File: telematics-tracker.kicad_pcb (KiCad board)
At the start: 4 copper layers, 82 x 62 mm, 216 parts, among them J1 WAFER-MX3.0-12PZZ, J2 B3B-XH-A, Q1 AM2390N-TP, Q10 MMBT3904, Q11 MMBT3904, Q12 MMBT3904, Q13 MMBT3906, Q14 MMBT3904, Q2 AM2390N-TP, Q3 AO3401A, Q4 MMBT3904, Q5 MMBT3904, Q6 MMBT3904, Q7 MMBT3904, Q8 MMBT3904, Q9 MMBT3904, U1 EC200UCNAA-N05-SGNSA, U2 AT32F403ACGT7, U3 QMI8658B, U4 SIT1051AT/3, U5 EG11752, U6 BQ25606RGER, U7 GD25Q64ESIGR, U8 TXB0104PWR, U9 ME6211C33M5G, X1 NANO-SIM, X2 MFF2-eSIM-pads, Y1 8MHz, Y2 32.768kHz

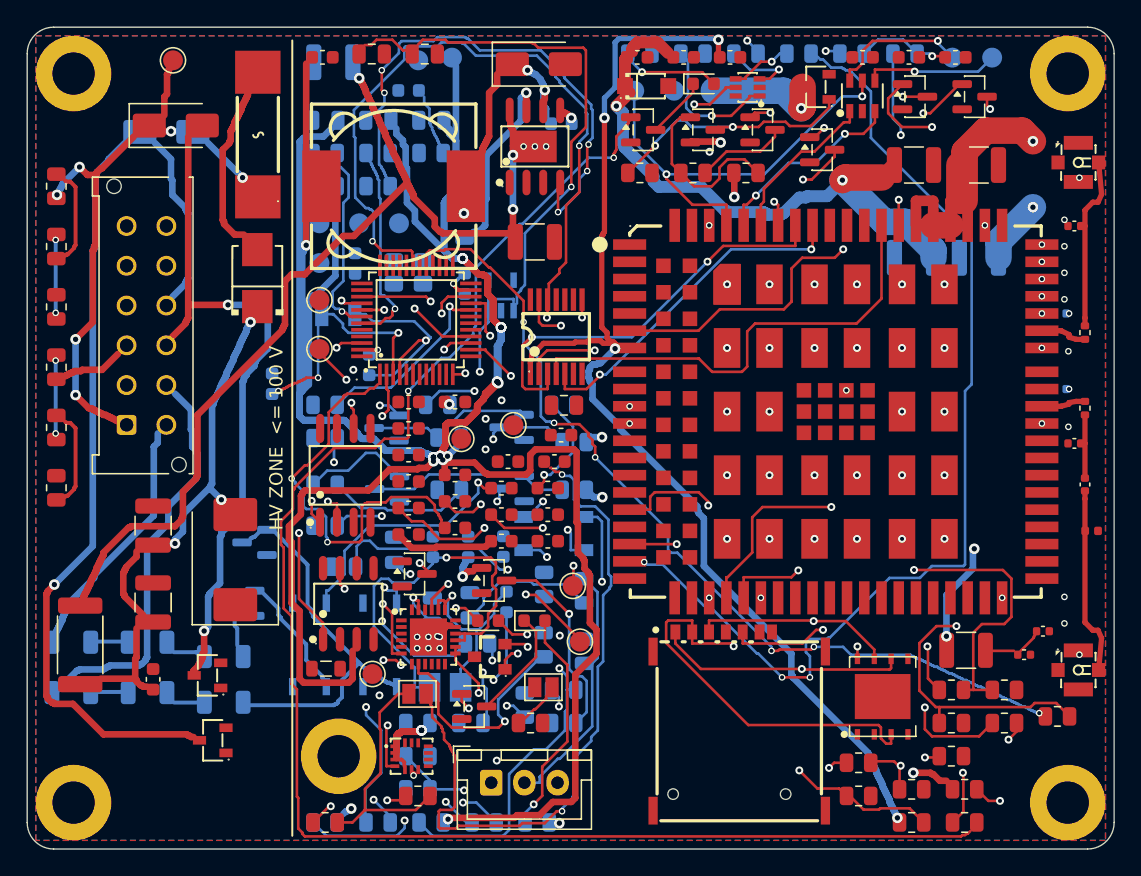
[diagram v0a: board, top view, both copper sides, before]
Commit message: hybrid v11 cycle 1: unconnected=150 errors=0
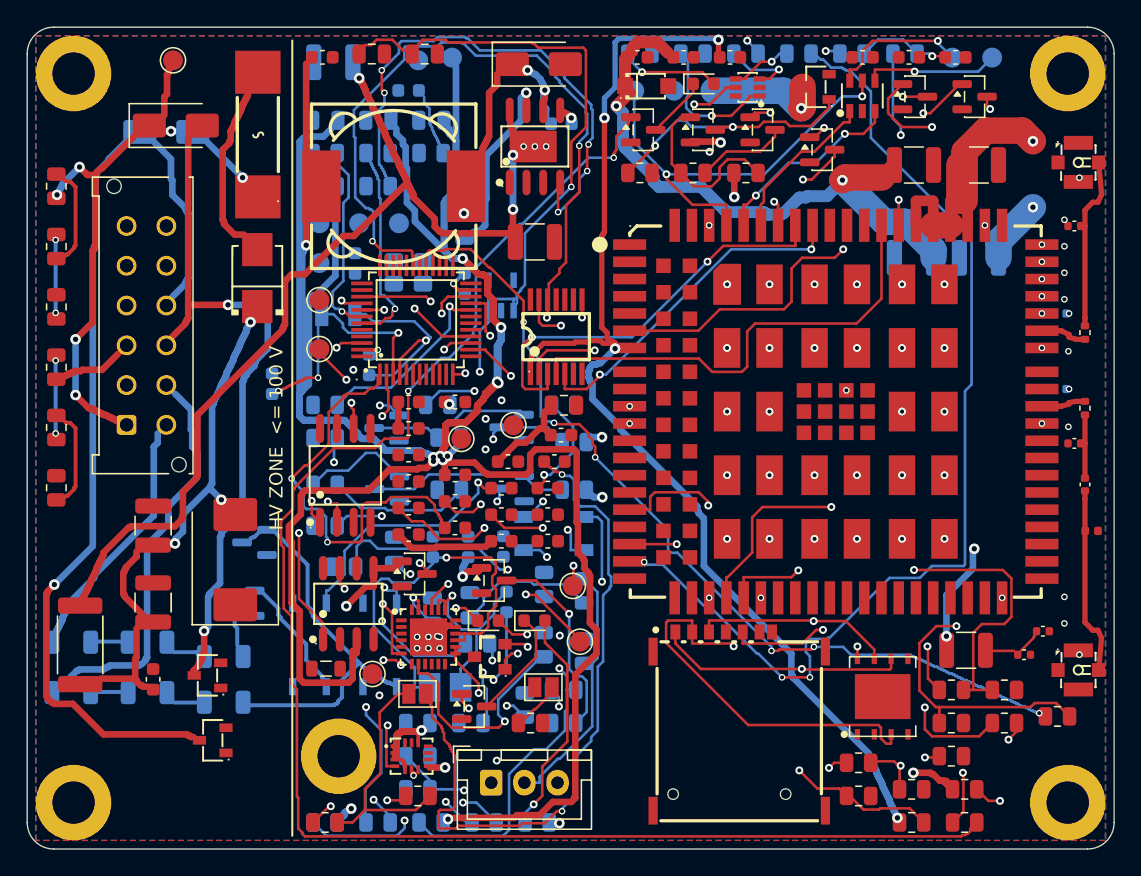
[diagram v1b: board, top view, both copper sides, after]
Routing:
- net 3V3: track 24.0 -> 54.1 mm
- net /modem_rf/VDD_EXT_1V8: track 86.2 -> 89.1 mm
- net 5V0: track 292.8 -> 294.7 mm, vias 22 -> 13
- net /mcu/BOOT0: track 2.42 -> 3.99 mm
- net /io/CAN_SPLIT: track 51.6 -> 53.1 mm
- net /mcu/VBAT_MCU: track 30.1 -> 31.5 mm
- net /modem_rf/Q12_B: track 120.4 -> 121.5 mm
- net /modem_rf/USIM_RST_M: track 77.6 -> 78.7 mm
- net /mcu/OSC32_IN: track 17.2 -> 18.3 mm
- net /mcu/I2C1_SDA: track 14.4 -> 15.1 mm
- net /mcu/I2C1_SCL: track 15.0 -> 15.7 mm
- net MODEM_PWRKEY: track 67.4 -> 68.0 mm
